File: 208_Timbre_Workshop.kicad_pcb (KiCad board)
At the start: 2 copper layers, 90.5 x 108.9 mm, 89 parts, among them J1 CV_IN, J2 AUDIO_IN, J3 AUDIO_OUT, J4 30310-6002HB, J5 Conn_01x05_Female, J6 Conn_01x05_Male, Q5 2N3905, Q6 2N4341, U1 TL072*, U2 TL084*, U3 TL084*

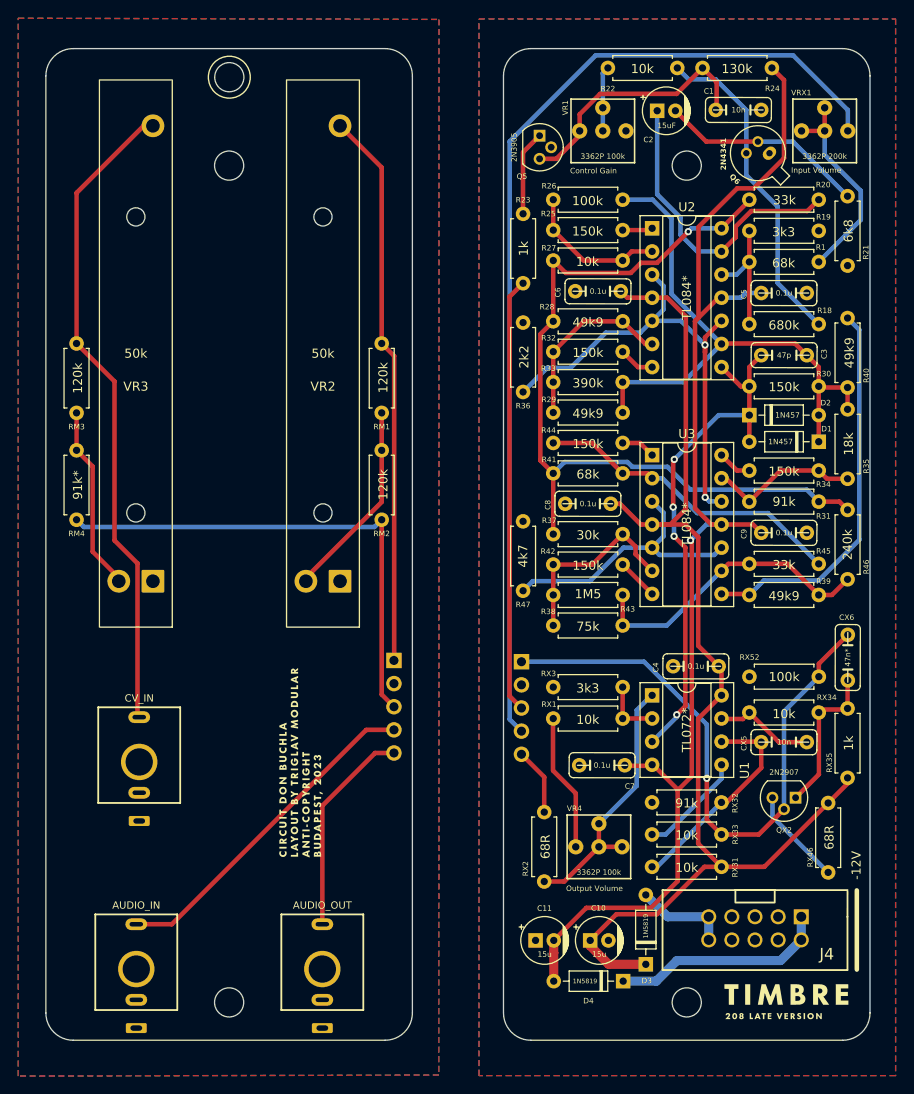
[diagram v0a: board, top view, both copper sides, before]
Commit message: Rev. 2
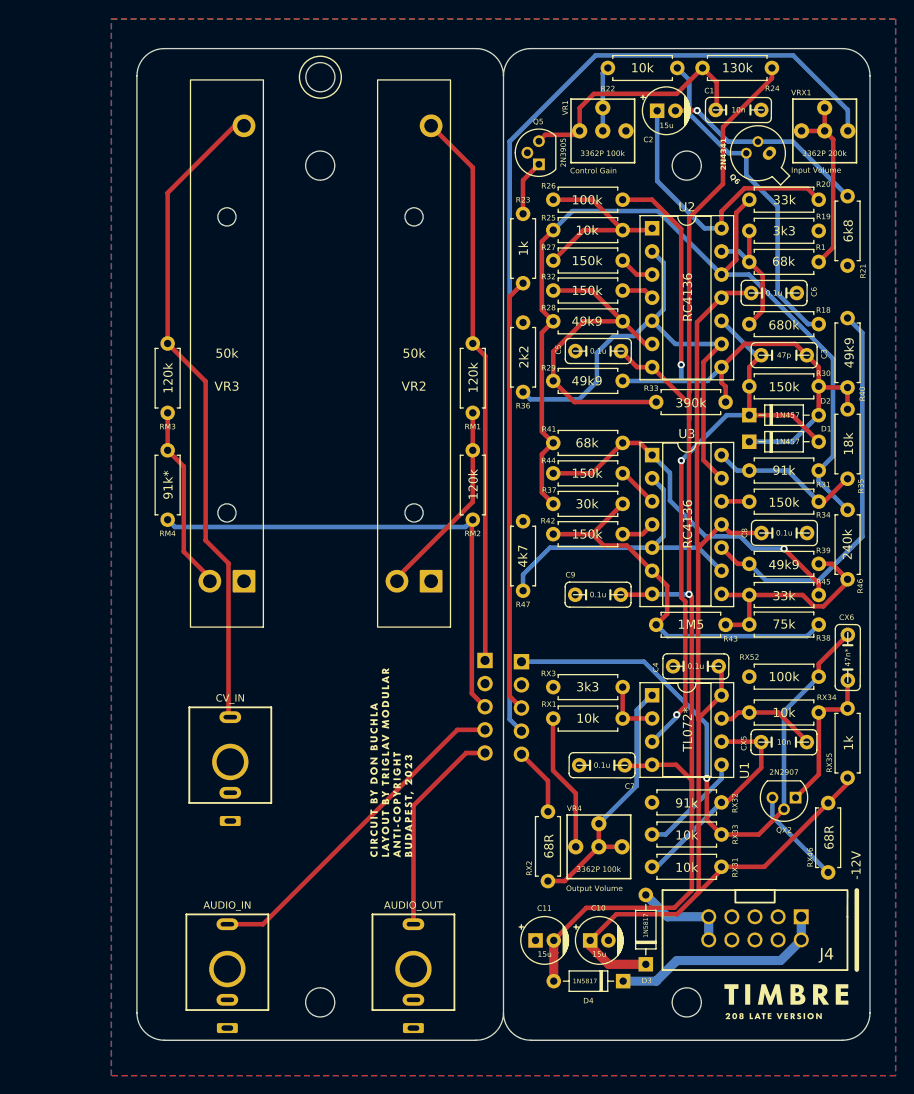
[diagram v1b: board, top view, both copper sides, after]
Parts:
- added G***: Rev2, Triglav_Modular:Rev2, B.Cu at (148.5, 136.7)
- added G***: Rev2, Triglav_Modular:Rev2, B.Cu at (177.5, 151.9)
- added G***: Rev2, Triglav_Modular:Rev2, B.Cu at (174.2, 109.7)
- C2: value 15uF -> 15u
- D3, D4: value 1N5819 -> 1N5817
- U2, U3: value TL084* -> RC4136
- moved C8 26.7 mm to (197.8, 98.2), turned to 180 degrees
- moved C6 24.3 mm to (196.7, 71.9), turned to 180 degrees
- moved R38 21.5 mm to (195.3, 108.3), turned to 180 degrees
- moved C9 16.9 mm to (177.4, 105.0), turned to 180 degrees
- moved C5 16.7 mm to (177.4, 78.3), turned to 180 degrees
- moved R43 11.8 mm to (185.1, 108.3)
- moved R33 11.5 mm to (185.1, 83.9)
- moved G*** 10.0 mm to (152.7, 110.2)
- moved G*** 10.0 mm to (144.4, 135.0)
- moved G*** 10.0 mm to (142.9, 104.5)
- moved J1 10.0 mm to (134.5, 123.4)
- moved J2 10.0 mm to (134.2, 146.1)
- moved J3 10.0 mm to (154.6, 146.1)
- moved J5 10.0 mm to (162.4, 112.2)
- moved REF** 10.0 mm to (144.4, 57.9)
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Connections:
- C1 pad 2: GND -> P_GND
- C10 pad 2: GND -> P_GND
- C11 pad 1: GND -> P_GND
- C4 pad 1: GND -> P_GND
- C5 pad 2: GND -> P_GND
- C6 pad 1: GND -> P_GND
- C7 pad 2: GND -> P_GND
- C8 pad 1: GND -> P_GND
- C9 pad 2: GND -> P_GND
- J4 pad 3: GND -> P_GND
- J4 pad 4: GND -> P_GND
- J4 pad 5: GND -> P_GND
- J4 pad 6: GND -> P_GND
- J4 pad 7: GND -> P_GND
- J4 pad 8: GND -> P_GND
- J6 pad 2: GND -> P_GND
- Q5 pad 2: GND -> P_GND
- Q6 pad 1: GND -> P_GND
- R19 pad 2: GND -> P_GND
- R21 pad 2: GND -> P_GND
- R36 pad 2: GND -> P_GND
- R47 pad 2: GND -> P_GND
- RX3 pad 1: GND -> P_GND
- RX32 pad 1: GND -> P_GND
- RX52 pad 1: GND -> P_GND
- U2 pad 1: Net-(R27-Pad1) -> Net-(U2A--)
- U2 pad 10: /GND2 -> Net-(D1-A)
- U2 pad 11: -12V -> +12V
- U2 pad 12: Net-(U2D-+) -> Net-(R20-Pad2)
- U2 pad 13: Net-(U2D--) -> Net-(U2D-+)
- U2 pad 14: Net-(R20-Pad2) -> Net-(U2D--)
- U2 pad 2: Net-(U2A--) -> /GND2
- U2 pad 3: /GND2 -> Net-(R27-Pad1)
- U2 pad 4: +12V -> Net-(R32-Pad1)
- U2 pad 7: Net-(R32-Pad1) -> -12V
- U2 pad 8: Net-(D1-A) -> Net-(D1-K)
- U2 pad 9: Net-(D1-K) -> /GND2
- U3 pad 1: Net-(R44-Pad1) -> Net-(U3A--)
- U3 pad 10: /GND3 -> Net-(R39-Pad2)
- U3 pad 11: -12V -> +12V
- U3 pad 12: /GND2 -> Net-(R34-Pad1)
- U3 pad 13: Net-(U3D--) -> /GND2
- U3 pad 14: Net-(R34-Pad1) -> Net-(U3D--)
- U3 pad 2: Net-(U3A--) -> /GND3
- U3 pad 3: /GND3 -> Net-(R44-Pad1)
- U3 pad 4: +12V -> Net-(R42-Pad1)
- U3 pad 7: Net-(R42-Pad1) -> -12V
- U3 pad 8: Net-(R39-Pad2) -> Net-(U3C--)
- U3 pad 9: Net-(U3C--) -> /GND3
- VR1 pad 3: GND -> P_GND
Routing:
- net Net-(U3B--): track 21.1 -> 43.2 mm
- net Net-(U2B--): track 19.9 -> 37.8 mm
- net Net-(D1-K): track 63.6 -> 72.4 mm, vias 0 -> 1
- net Net-(U3C--): track 33.0 -> 25.0 mm
- net Net-(R20-Pad2): track 91.6 -> 99.5 mm, vias 1 -> 0
- net Net-(D1-A): track 57.3 -> 64.0 mm, vias 4 -> 2
- net -12V: track 140.6 -> 146.4 mm
- net Net-(U3A--): track 34.6 -> 40.0 mm, vias 0 -> 1
- net Net-(U2A--): track 16.0 -> 21.0 mm
- net /GND3: track 30.5 -> 34.5 mm
- net Net-(Q5-E): track 9.33 -> 6.16 mm
- net Net-(U2D--): track 33.7 -> 31.0 mm
- net Net-(R1-Pad1): track 23.0 -> 20.5 mm
- net Net-(R39-Pad2): track 42.4 -> 43.6 mm
- net Net-(U2D-+): track 13.9 -> 15.0 mm
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- removed copper zone on B.Cu, net GND
- removed copper zone on F.Cu, net GND
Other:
- board size 90.5 x 108.9 mm -> 80.5 x 108.9 mm
- board text added: "HEADER ON THIS SIDE"
